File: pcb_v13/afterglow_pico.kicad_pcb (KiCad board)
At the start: 2 copper layers, 57.5 x 100 mm, 52 parts, among them J1 Conn_02x17_Odd_Even, J2 Conn_02x17_Odd_Even, J3 Conn_01x02_Male, U1 74LS21, U2 7408, U3 SN74LVC245AN, U4 SN74LVC245AN, U5 Raspberry Pi Pico, U6 74LS245, U7 74LS245, U8 74LS257, U9 74LS257

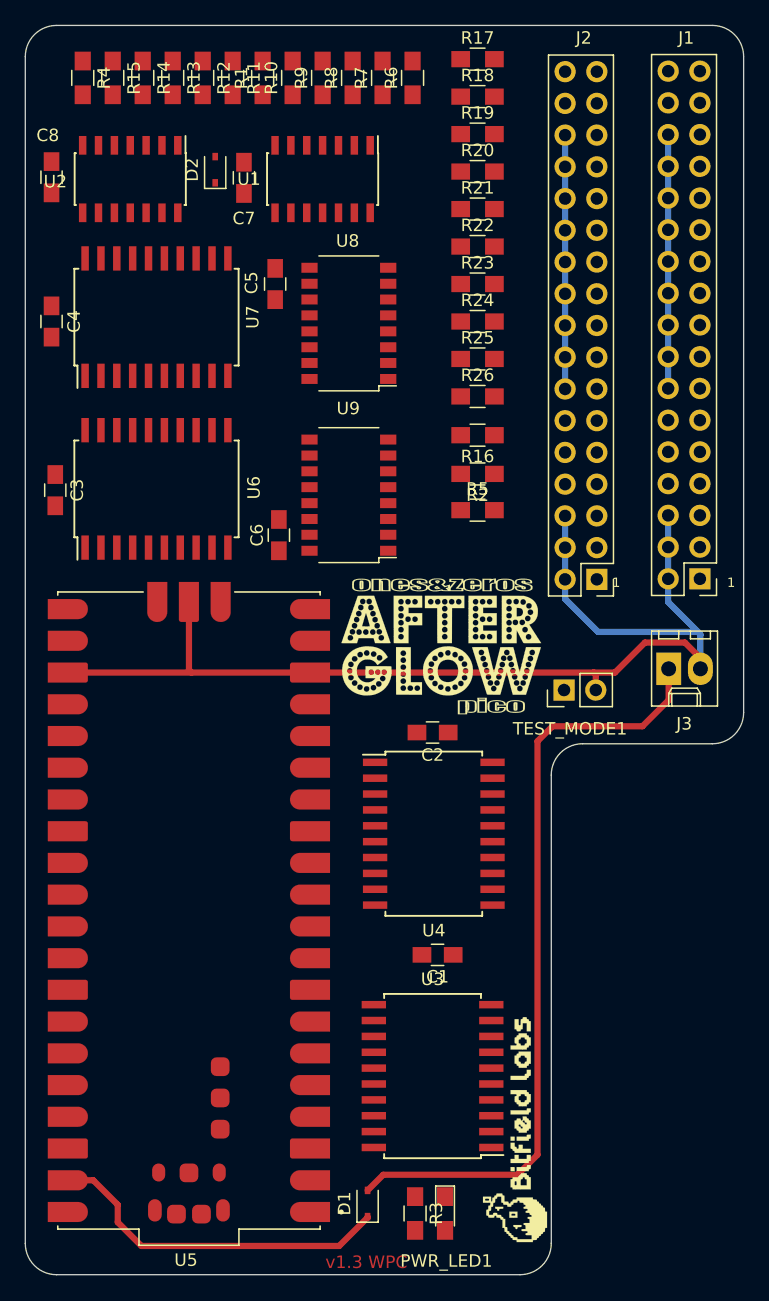
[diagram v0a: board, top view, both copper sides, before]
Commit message: First PCB v1.3 draft
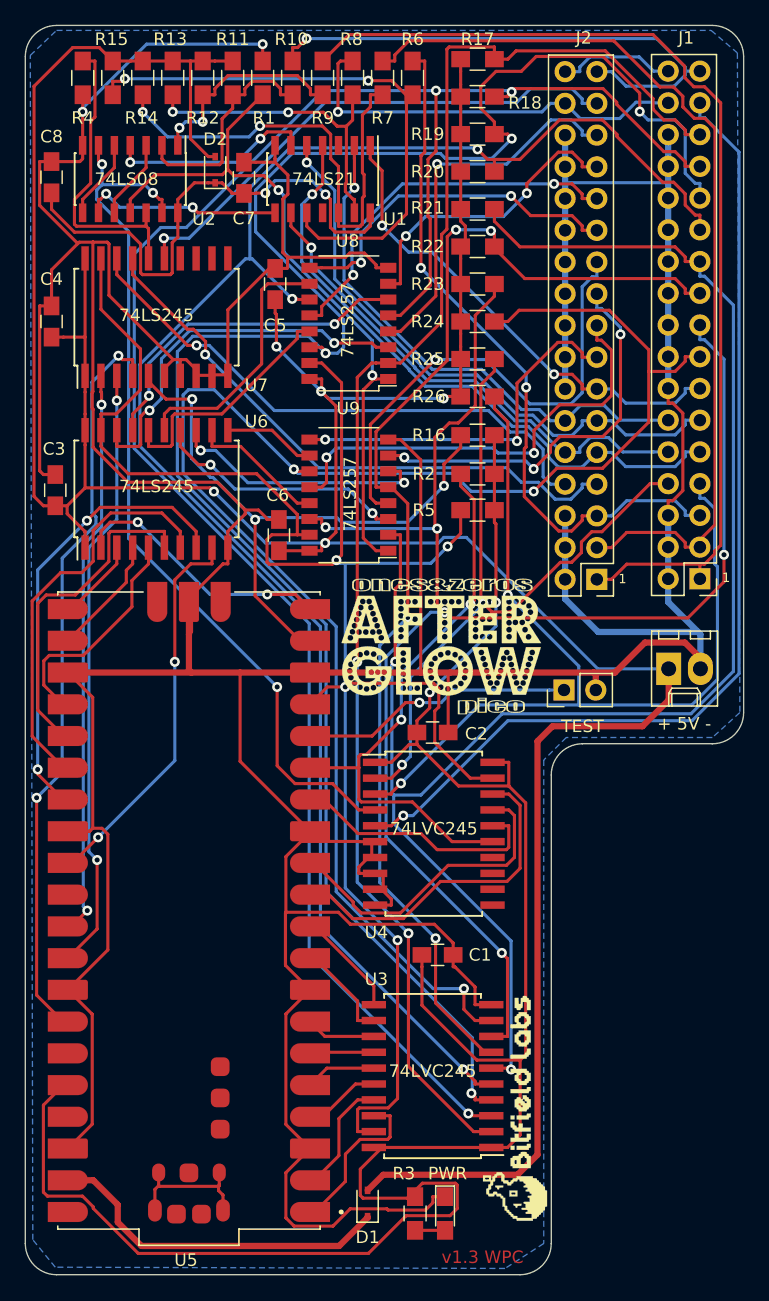
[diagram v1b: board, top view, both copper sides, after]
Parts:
- added G***: LOGO, pcb_v13:qr_code, B.Cu at (170.5, 129.9)
- + 5V -: renamed from J3
- moved BFL_LOGO 1.70 mm to (196.7, 132.3)
- renumbered PWR_LED1 to PWR, TEST_MODE1 to TEST
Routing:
- net GND: track 132.6 -> 481.6 mm, vias 0 -> 2
- net +5V: track 62.2 -> 271.4 mm, vias 0 -> 5
- net +3V3: track 0.00 -> 159.4 mm, vias 0 -> 2
- net /D2: track 0.00 -> 157.9 mm, vias 0 -> 4
- net /D1: track 0.00 -> 157.4 mm, vias 0 -> 3
- net /PICO_EN_OUT: track 0.00 -> 152.3 mm, vias 0 -> 4
- net /D3: track 0.00 -> 139.1 mm, vias 0 -> 3
- net /D4: track 0.00 -> 134.0 mm, vias 0 -> 2
- net /D7: track 0.00 -> 131.6 mm, vias 0 -> 3
- net /D6: track 0.00 -> 126.9 mm, vias 0 -> 5
- net /D0: track 0.00 -> 121.3 mm, vias 0 -> 2
- net /D5: track 0.00 -> 97.8 mm, vias 0 -> 4
- net /DIS_STROBE: track 0.00 -> 83.3 mm
- net /BLANK: track 0.00 -> 81.4 mm, vias 0 -> 1
- net /LROW: track 0.00 -> 75.2 mm, vias 0 -> 2
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- added copper zone on B.Cu, net GND
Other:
- board text added: "74LS08"
- board text added: "74LS21"
- board text added: "74LS245"
- board text added: "74LS257"
- board text added: "74LVC245"
